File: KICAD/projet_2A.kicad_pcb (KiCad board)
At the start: 2 copper layers, 6 parts, among them IC1 TPA3116D2QDADRQ1, IC2 TPA3116D2QDADRQ1, IC3 PCM1808PW, IC4 PCM5102AQPWRQ1, IC5 STM32F746BGT6, U1 FSC-BT1026E

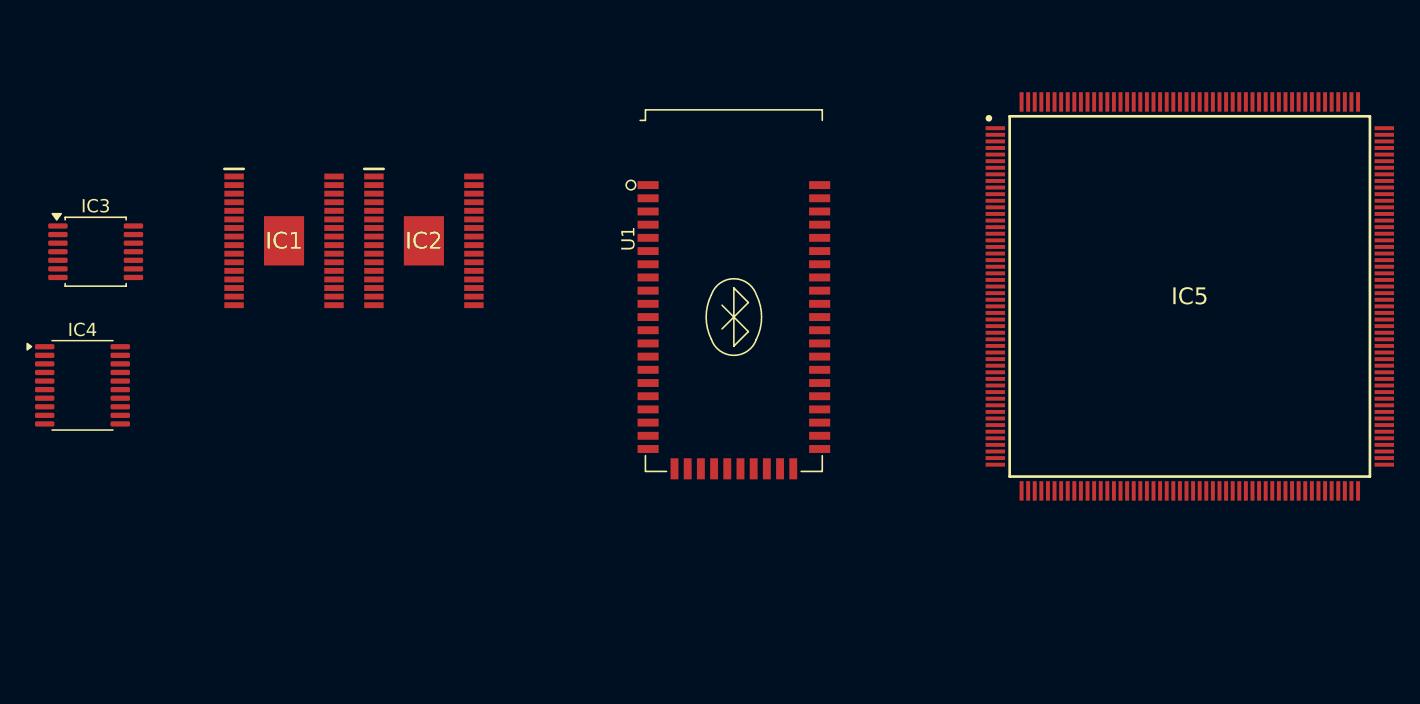
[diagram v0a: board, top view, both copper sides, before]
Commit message: BT + PCM1808
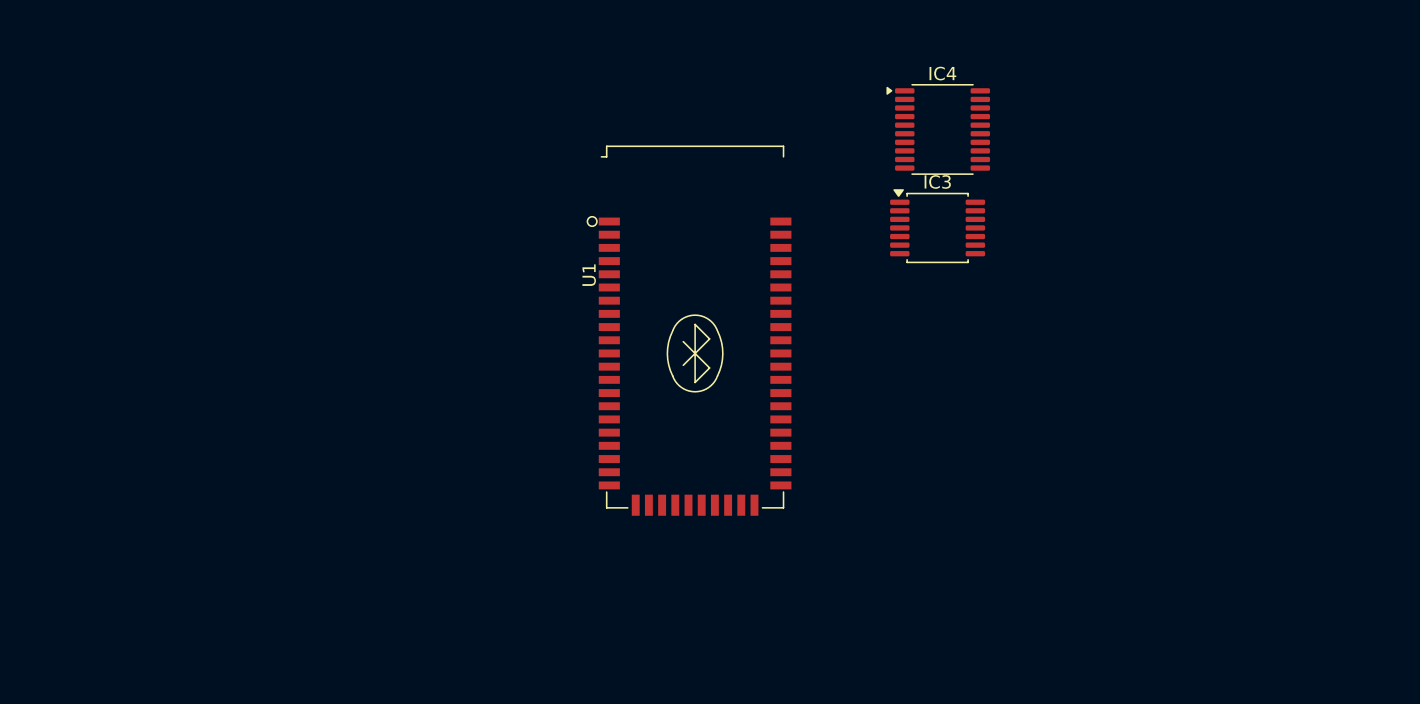
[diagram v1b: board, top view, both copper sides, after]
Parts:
- removed IC1, IC2: TPA3116D2QDADRQ1, TPA3116D2QDADRQ1:SOP65P810X120-33N
- removed IC5: STM32F746BGT6, STM32F746BGT6:QFP50P3000X3000X160-208N
- moved IC4 68.0 mm to (186.5, 74.1)
- moved IC3 63.8 mm to (186.1, 81.5)
- moved U1 4.03 mm to (167.8, 91.1)

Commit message: clear
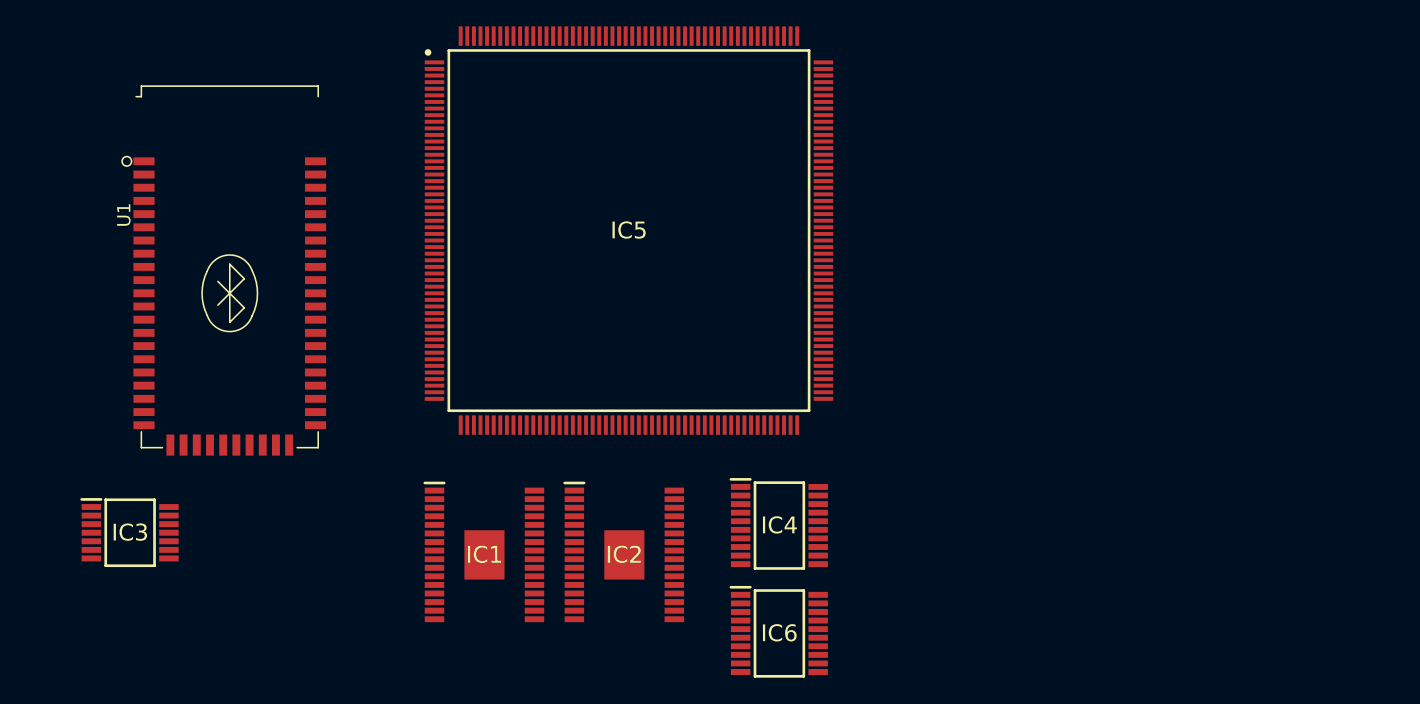
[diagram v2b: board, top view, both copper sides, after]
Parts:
- added IC1: TPA3116D2QDADRQ1, footprints:TPA3116D2QDADRQ1, F.Cu at (151.8, 106.3)
- added IC2: TPA3116D2QDADRQ1, footprints:TPA3116D2QDADRQ1, F.Cu at (162.4, 106.3)
- added IC5: STM32F746BGT6, footprints:STM32F746BGT6, F.Cu at (162.8, 81.8)
- added IC6: PCM5102AQPWRQ1, footprints:PCM5102AQPWRQ1, F.Cu at (174.2, 112.3)
- IC3: footprint Package_SO:TSSOP-14_4.4x5mm_P0.65mm -> footprints:PCM1808PW
- IC4: footprint Package_SO:TSSOP-20_4.4x6.5mm_P0.65mm -> footprints:PCM5102AQPWRQ1
- U1: footprint Bluetooth:FSC-BT1026x -> footprints:FSC-BT1026x
- moved IC3 65.4 mm to (125.0, 104.6)
- moved U1 35.6 mm to (132.5, 86.5)
- moved IC4 32.5 mm to (174.2, 104.1)
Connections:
- IC3 pad 1: unconnected-(IC3-VREF-Pad1) -> Net-(IC3-VREF)
- IC3 pad 10: unconnected-(IC3-MD0-Pad10) -> GND
- IC3 pad 11: unconnected-(IC3-MD1-Pad11) -> GND
- IC3 pad 12: unconnected-(IC3-FMT-Pad12) -> GND
- IC3 pad 13: unconnected-(IC3-VINL-Pad13) -> Net-(IC3-VINL)
- IC3 pad 14: unconnected-(IC3-VINR-Pad14) -> Net-(IC3-VINR)
- IC3 pad 2: unconnected-(IC3-AGND-Pad2) -> GND
- IC3 pad 3: unconnected-(IC3-VCC-Pad3) -> +5V
- IC3 pad 4: unconnected-(IC3-VDD-Pad4) -> +3.3V
- IC3 pad 5: unconnected-(IC3-DGND-Pad5) -> GND
- IC3 pad 6: unconnected-(IC3-SCKI-Pad6) -> /ADC_PCM1808/SCKI/SAI1_MCLK_A
- IC3 pad 7: unconnected-(IC3-LRCK-Pad7) -> /ADC_PCM1808/LRCK/SAI1_FS_A
- IC3 pad 8: unconnected-(IC3-BCK-Pad8) -> /ADC_PCM1808/BCK/SAI1_SCK_A
- IC3 pad 9: unconnected-(IC3-DOUT-Pad9) -> /ADC_PCM1808/DOUT/SAI1_SD_A
- IC4 pad 1: unconnected-(IC4-CPVDD-Pad1) -> +3.3VA
- IC4 pad 10: unconnected-(IC4-DEMP-Pad10) -> GND
- IC4 pad 11: unconnected-(IC4-FLT-Pad11) -> GND
- IC4 pad 12: unconnected-(IC4-SCK-Pad12) -> GND
- IC4 pad 13: unconnected-(IC4-BCK-Pad13) -> /ADC_PCM1808/BCK/SAI1_SCK_A
- IC4 pad 14: unconnected-(IC4-DIN-Pad14) -> /DAC_PCM5102A/DIN/SAI1_SD_A
- IC4 pad 15: unconnected-(IC4-LRCK-Pad15) -> /ADC_PCM1808/LRCK/SAI1_FS_A
- IC4 pad 16: unconnected-(IC4-FMT-Pad16) -> GND
- IC4 pad 17: unconnected-(IC4-XSMT-Pad17) -> Net-(IC4-XSMT)
- IC4 pad 18: unconnected-(IC4-LDOO-Pad18) -> Net-(IC4-LDOO)
- IC4 pad 19: unconnected-(IC4-DGND-Pad19) -> GND
- IC4 pad 2: unconnected-(IC4-CAPP-Pad2) -> Net-(IC4-CAPP)
- IC4 pad 20: unconnected-(IC4-DVDD-Pad20) -> +3.3V
- IC4 pad 3: unconnected-(IC4-CPGND-Pad3) -> GND
- IC4 pad 4: unconnected-(IC4-CAPM-Pad4) -> Net-(IC4-CAPM)
- IC4 pad 5: unconnected-(IC4-VNEG-Pad5) -> Net-(IC4-VNEG)
- IC4 pad 6: unconnected-(IC4-OUTL-Pad6) -> Net-(IC4-OUTL)
- IC4 pad 7: unconnected-(IC4-OUTR-Pad7) -> Net-(IC4-OUTR)
- IC4 pad 8: unconnected-(IC4-AVDD-Pad8) -> +3.3VA
- IC4 pad 9: unconnected-(IC4-AGND-Pad9) -> GND
- U1 pad 1: Net-(U1-GND-Pad1) -> GND
- U1 pad 13: unconnected-(U1-BT_TX/PI05-Pad13) -> /Bluetooth/USART_TX
- U1 pad 14: unconnected-(U1-BT_RX/PI04-Pad14) -> /Bluetooth/USART_RX
- U1 pad 22: Net-(U1-GND-Pad1) -> GND
- U1 pad 32: Net-(U1-GND-Pad1) -> GND
- U1 pad 33: unconnected-(U1-VBAT_IN-Pad33) -> +3.3V
- U1 pad 34: unconnected-(U1-SYS_CTRL-Pad34) -> +3.3V
- U1 pad 36: unconnected-(U1-VDD_IO-Pad36) -> +3.3V
- U1 pad 46: unconnected-(U1-AUDIO_HPR_N-Pad46) -> GND
- U1 pad 47: unconnected-(U1-AUDIO_HPR_P-Pad47) -> /Bluetooth/AUDIO_HPR_P
- U1 pad 48: unconnected-(U1-AUDIO_HPL_N-Pad48) -> GND
- U1 pad 49: unconnected-(U1-AUDIO_HPL_P-Pad49) -> /Bluetooth/AUDIO_HPL_P
- U1 pad 50: Net-(U1-GND-Pad1) -> GND
- U1 pad 52: Net-(U1-GND-Pad1) -> GND
- U1 pad 8: unconnected-(U1-RESET-Pad8) -> Net-(U1-RESET)
